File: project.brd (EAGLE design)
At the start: 88.9 x 75.7 mm, 58 parts, among them IC1 ADP3338AKCZ-5-R7, J1 22-23-2021, Y1 ABM8-20.000MHZ-B2-T

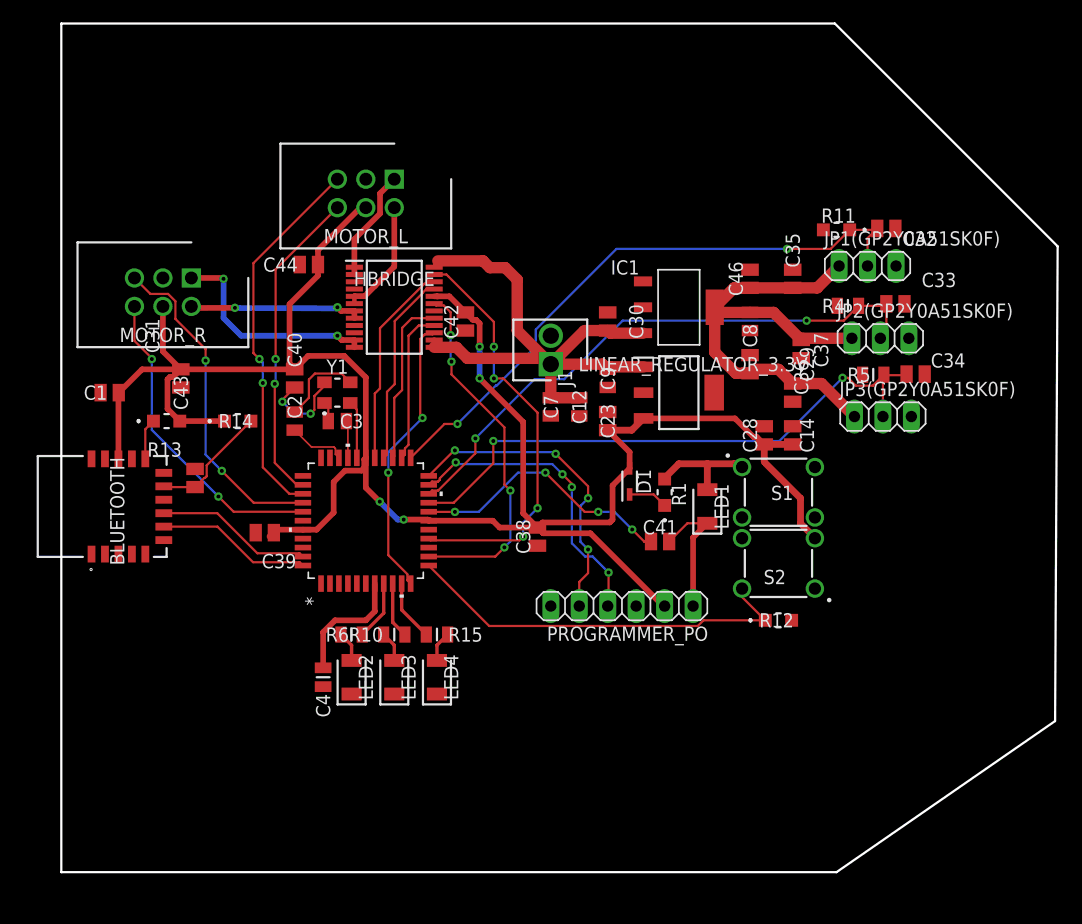
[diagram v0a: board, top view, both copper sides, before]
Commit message: review #1
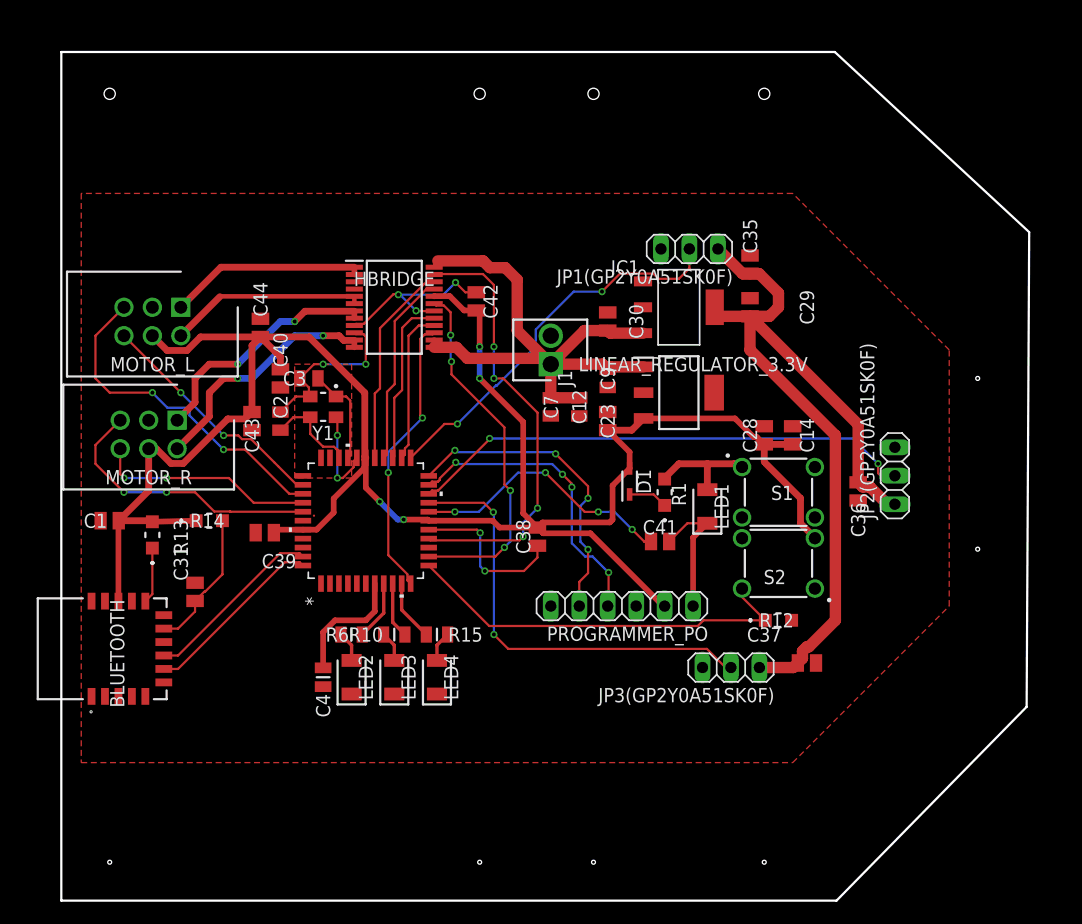
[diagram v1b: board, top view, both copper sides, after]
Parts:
- removed C32, C33, C34, C46: C0805J104K1RACAUTO, C0805J104K1RACAUTO:CAPC2012X140N
- removed C8: 0805YC106KAT2A, 0805YC106KAT2A:CAPC2012X94N
- removed R11: ERA-6ARW472V, ERA-6ARW472V:ERA6AEB101V
- removed R4, R5: RNCE0805BTE10K0, RNCE0805BTE10K0:RESC2012X65N
- moved JP3(GP2Y0A51SK0F) 26.2 mm to (87.2, 30.1), turned to 180 degrees
- moved C37 24.2 mm to (94.0, 30.5), turned to 0 degrees
- moved MOTOR_L 22.2 mm to (38.1, 62.2)
- moved JP1(GP2Y0A51SK0F) 16.0 mm to (83.5, 67.4), turned to 180 degrees
- moved C36 13.7 mm to (98.6, 45.8)
- moved MOTOR_R 12.8 mm to (37.8, 52.1)
- moved BLUETOOTH 12.7 mm to (36.8, 31.8)
- moved JP2(GP2Y0A51SK0F) 12.3 mm to (101.8, 47.2), turned to 90 degrees
- moved C1 11.4 mm to (31.8, 43.2)
- moved R13 10.2 mm to (35.6, 41.9), turned to 90 degrees
- moved C31 10.2 mm to (39.4, 36.8)
- moved R14 9.25 mm to (40.6, 43.2)
- moved C43 7.41 mm to (44.5, 52.1)
- moved C44 7.11 mm to (45.2, 60.4), turned to 90 degrees
- moved C29 5.08 mm to (88.9, 62.2)
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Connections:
- removed net N$3: C3.1, Y1.1
- removed net N$4: C2.2, Y1.3
- net 5V: no longer C46.1, C8.1
- net AN0: no longer C33.1, R4.1
- net AN1: no longer C34.1, R5.1
- net AN4: no longer C32.1, R11.1
- net BO1: now also MOTOR_R.2; no longer MOTOR_R.1
- net BO2: now also MOTOR_R.1; no longer MOTOR_R.2
- net ENCR_A: now also MICROCHIP.38; no longer MICROCHIP.37
- net ENCR_B: now also MICROCHIP.37; no longer MICROCHIP.38
- net GND: now also C2.2, C3.2; no longer C32.2, C33.2, C34.2, C46.2, C8.2, R11.2, R4.2, R5.2
- net N$1: now also Y1.3
- net N$2: now also C3.1, Y1.1; no longer C3.2
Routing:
- net GND: track 13.1 -> 55.5 mm, vias 2 -> 9
- net 5V: track 45.3 -> 77.2 mm
- net AN4: track 54.7 -> 34.9 mm
- net AN1: track 53.0 -> 39.4 mm
- net ENCR_B: track 28.2 -> 19.6 mm
- net N$4: track 7.66 -> 0.00 mm
- net AO1: track 9.98 -> 17.6 mm
- net AO2: track 10.6 -> 17.6 mm
- net ENCL_B: track 28.4 -> 21.5 mm
- net AN0: track 51.9 -> 45.6 mm
- net BO2: track 15.4 -> 21.7 mm
- net N$2: track 3.33 -> 8.89 mm
- net ENCR_A: track 29.8 -> 25.1 mm
- net ENCL_A: track 33.7 -> 30.5 mm
- net N$1: track 5.27 -> 8.42 mm
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- added copper zone on layer 1, net GND
- added copper zone on layer 1, net GND_EXC
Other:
- board size 88.9 x 75.7 mm -> 86.4 x 75.7 mm

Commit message: Fertig?
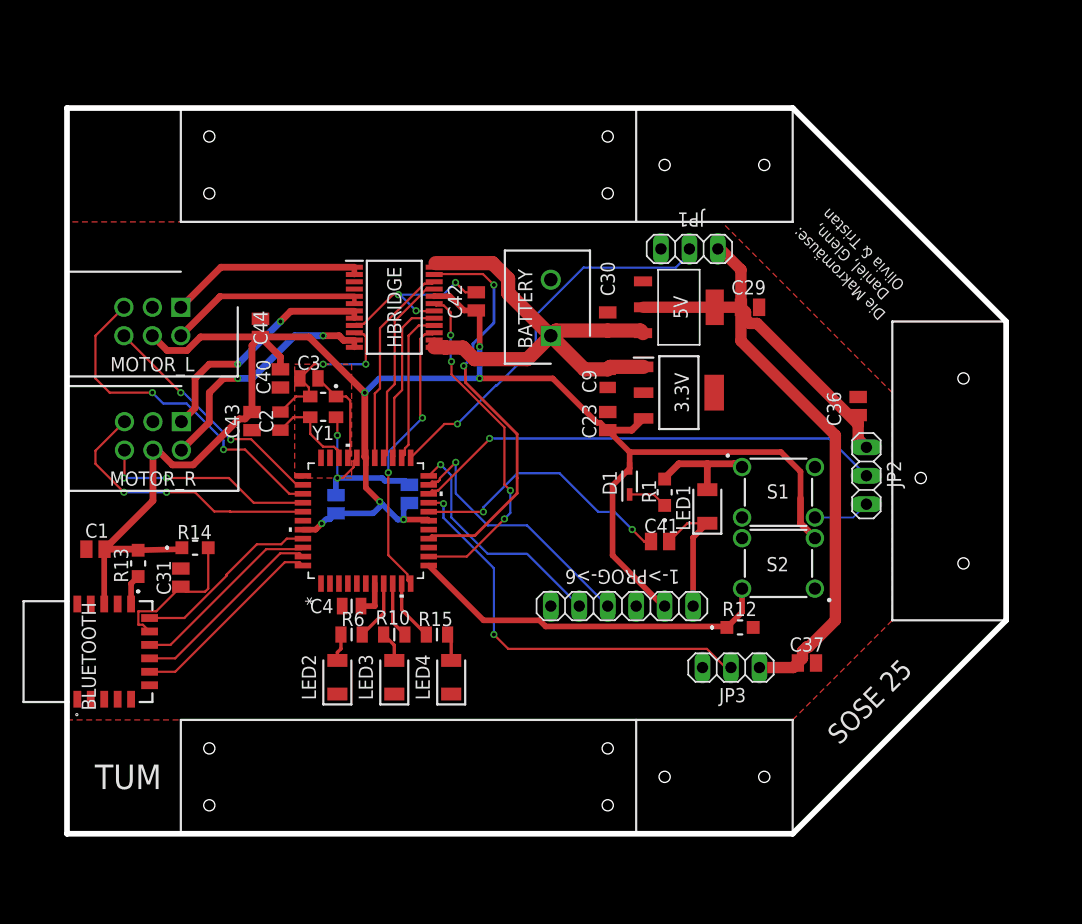
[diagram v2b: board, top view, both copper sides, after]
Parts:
- removed C12, C7: 0805YC106KAT2A, 0805YC106KAT2A:CAPC2012X94N
- removed C14, C28, C35: C0805J104K1RACAUTO, C0805J104K1RACAUTO:CAPC2012X140N
- removed J1: 22-23-2021, 22-23-2021:SHDR2W87P0X254_1X2_493X635X110
- removed JP2(GP2Y0A51SK0F): (no value), pinhead:1X03
- added BATTERY: 691137710002, 691137710002:SHDR2W70P0X500_1X2_1000X750X11
- added JP2: (no value), pinhead:1X03
- moved C38 12.0 mm to (58.5, 45.6), flipped to the bottom, turned to 90 degrees
- moved C36 7.62 mm to (98.6, 53.4), turned to 90 degrees
- moved C4 6.84 mm to (53.3, 35.6), turned to 0 degrees
- moved C39 6.84 mm to (51.9, 44.7), flipped to the bottom, turned to 90 degrees
- moved R12 3.49 mm to (88.0, 33.7)
- moved R13 2.84 mm to (34.3, 39.4)
- moved C1 2.84 mm to (30.5, 40.6)
- moved R14 2.73 mm to (39.4, 40.8)
- moved C31 1.80 mm to (38.1, 38.1)
- moved BLUETOOTH 1.30 mm to (35.6, 31.5)
- moved LED2 1.27 mm to (52.1, 29.2)
- moved LED4 1.27 mm to (62.2, 29.2)
- moved MOTOR_R 0.40 mm to (38.2, 52.0)
- turned C29 to 0 degrees
- renumbered IC1 to 5V, JP1(GP2Y0A51SK0F) to JP1, JP3(GP2Y0A51SK0F) to JP3, LINEAR_REGULATOR_3.3V to 3.3V, PROGRAMMER_PO to 1->PROG->6
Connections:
- net 3.3V: no longer C14.1, C28.1
- net 5V: now also 5V.2, JP2.1; no longer C35.1, JP2(GP2Y0A51SK0F).1
- net AN0: now also JP2.2; no longer JP2(GP2Y0A51SK0F).2
- net CTS: now also MICROCHIP.41
- net GND: now also BATTERY.2, JP2.3; no longer C12.2, C14.2, C28.2, C35.2, C7.2, J1.2, JP2(GP2Y0A51SK0F).3
- net RTS: now also MICROCHIP.42
- net VM: now also BATTERY.1; no longer C12.1, C7.1, J1.1
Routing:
- net RTS: track 0.00 -> 17.3 mm
- net 3.3V: track 188.3 -> 171.5 mm, vias 4 -> 6
- net CTS: track 0.00 -> 16.7 mm
- net VM: track 52.6 -> 44.6 mm
- net N$7: track 11.0 -> 3.24 mm
- net PGEC1: track 28.1 -> 21.3 mm, vias 4 -> 1
- net 5V: track 77.2 -> 73.6 mm
- net PGED1: track 27.2 -> 23.8 mm, vias 4 -> 1
- net N$16: track 36.2 -> 32.9 mm
- net AN0: track 45.6 -> 42.5 mm, vias 2 -> 1
- net N$27: track 5.00 -> 2.71 mm
- net PWM_L: track 39.5 -> 37.3 mm, vias 4 -> 2
- net AN1: track 39.4 -> 37.3 mm
- net GND: track 55.5 -> 53.8 mm, vias 9 -> 7
- net STBY: track 32.3 -> 30.8 mm
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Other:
- board size 86.4 x 75.7 mm -> 83.8 x 64.8 mm
- board text added: "Die Makromäuse: Daniel, Glenn, Olivia & Tristan"
- board text added: "SOSE 25"
- board text added: "TUM"
